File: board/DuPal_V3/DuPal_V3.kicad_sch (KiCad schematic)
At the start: 128 parts, among them J1 ZIF Socket, J2 Debug Header, K1 G6K-2, Q1 2N3904, SW1 RESET, U1 Pico, U10 74HCT166, U11 74HCT166, U12 74HCT166, U13 SN74LV1T125DBV, U2 74HCT595, U3 74HCT595, U4 74HCT595, U5 74HCT595, U6 74HCT595, U7 74HCT02, U8 74HCT166, U9 74HCT166

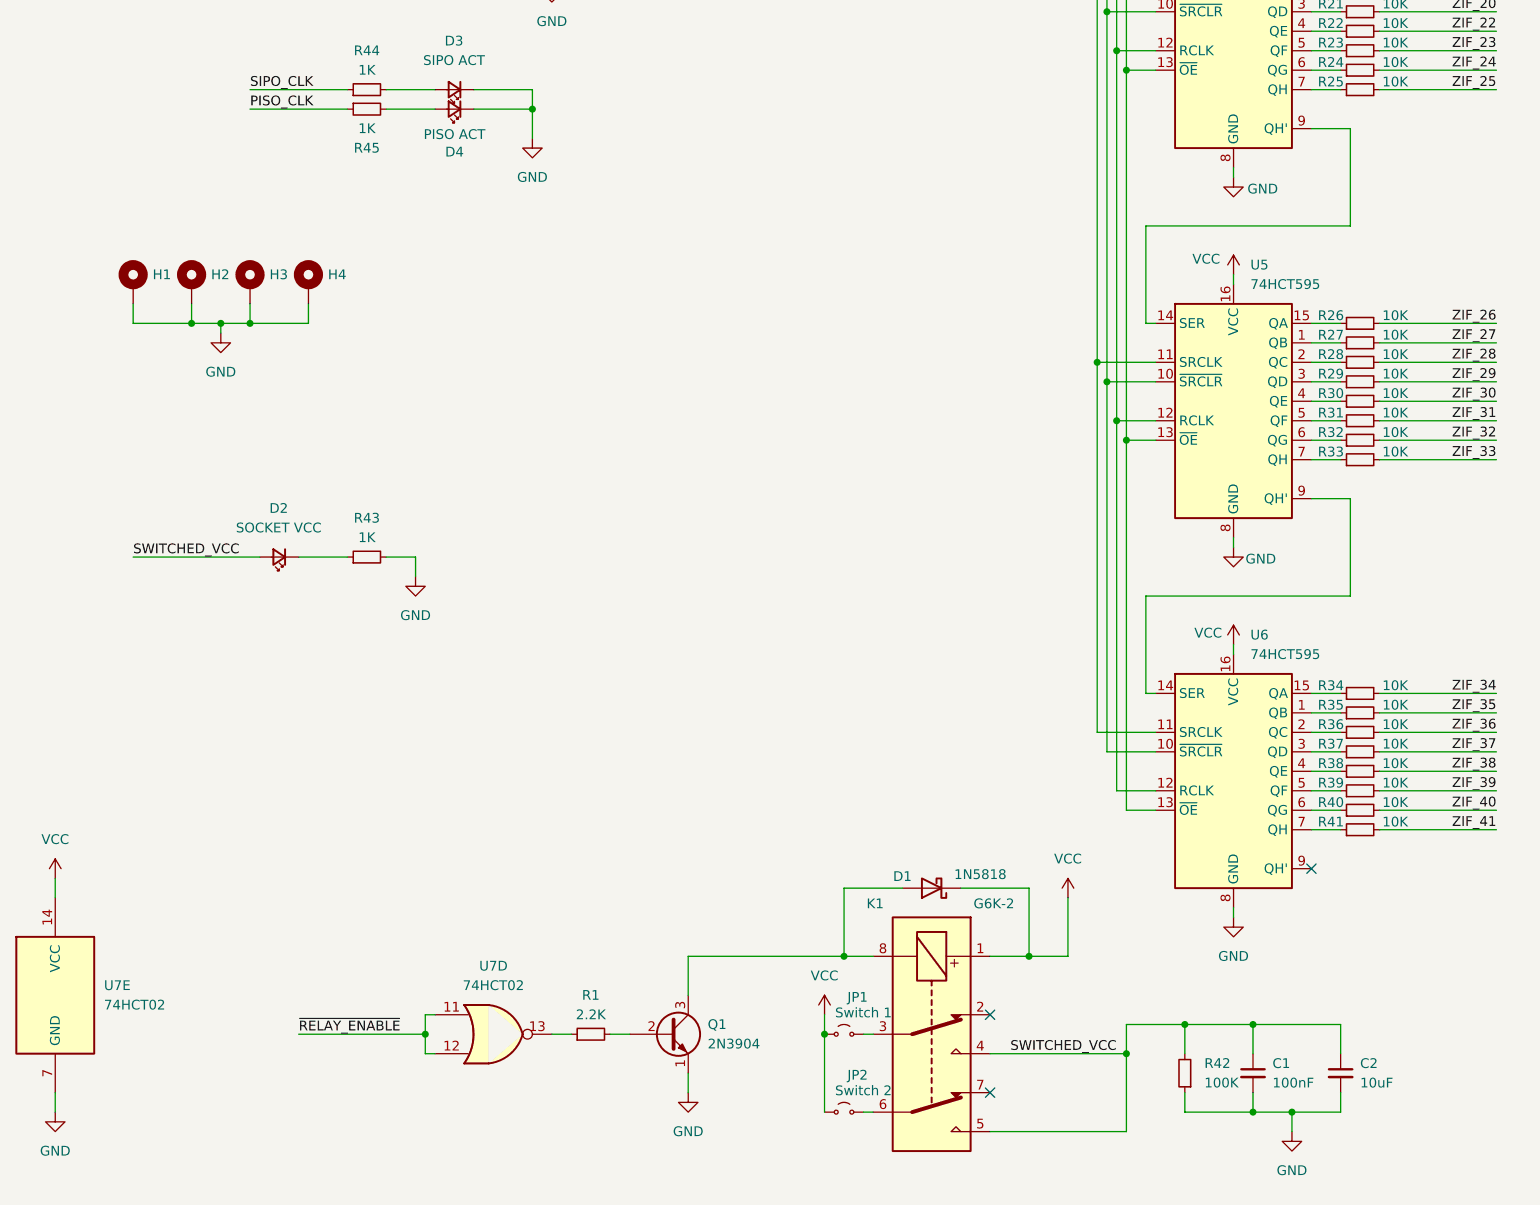
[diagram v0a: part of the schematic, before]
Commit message: Cleanup
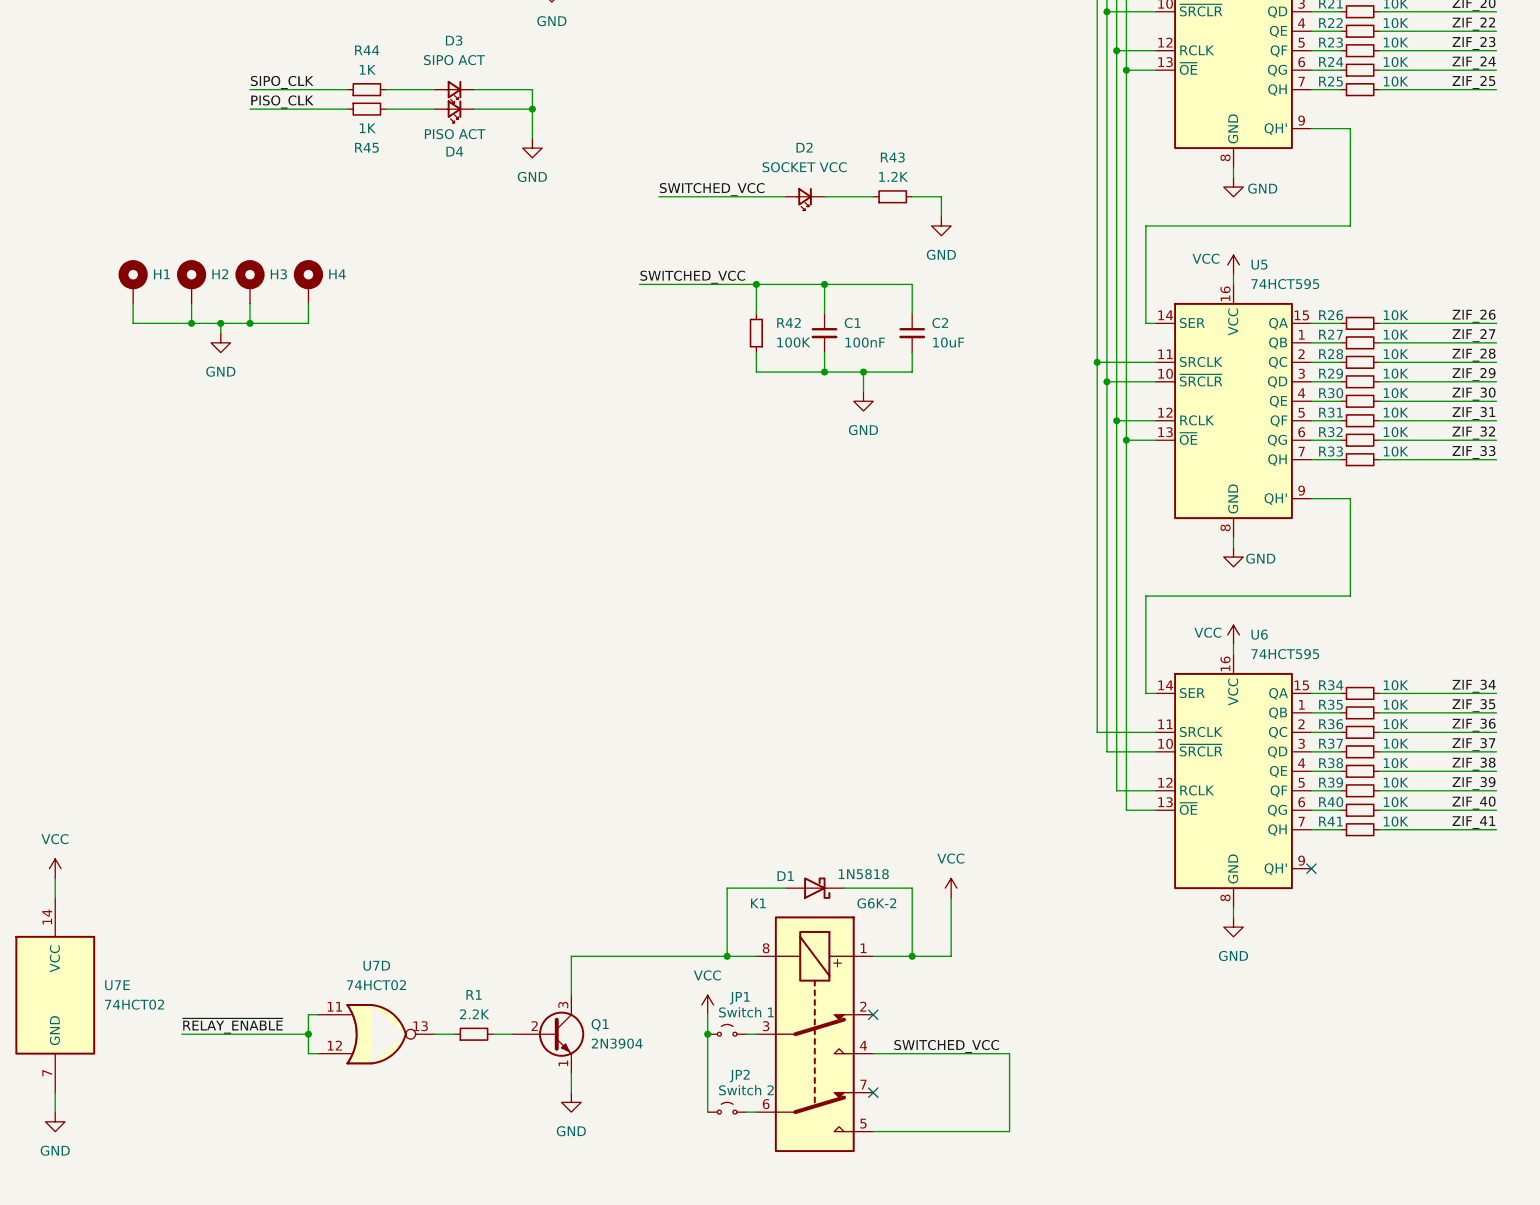
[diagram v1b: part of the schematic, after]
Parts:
- R43: value 1K -> 1.2K
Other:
- moved on the sheet: C1, C2, D1, D2, JP1, JP2, K1, Q1, R1, R42, R43, U7D
